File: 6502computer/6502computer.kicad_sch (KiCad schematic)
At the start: 28 parts

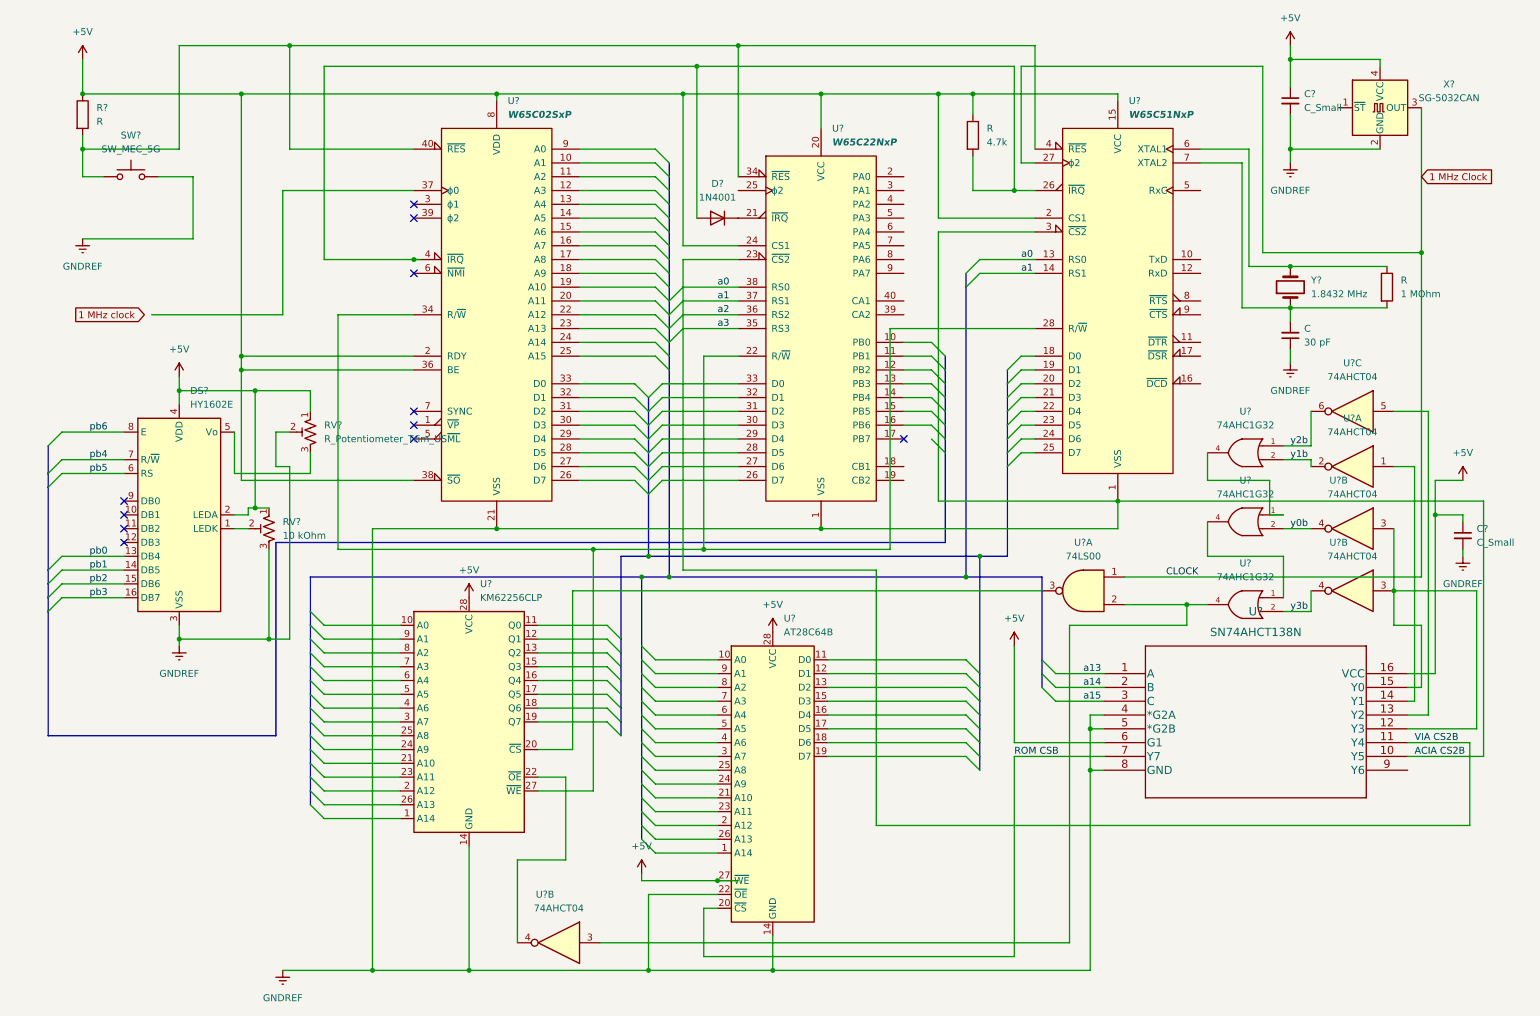
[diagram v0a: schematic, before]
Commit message: Update schematics
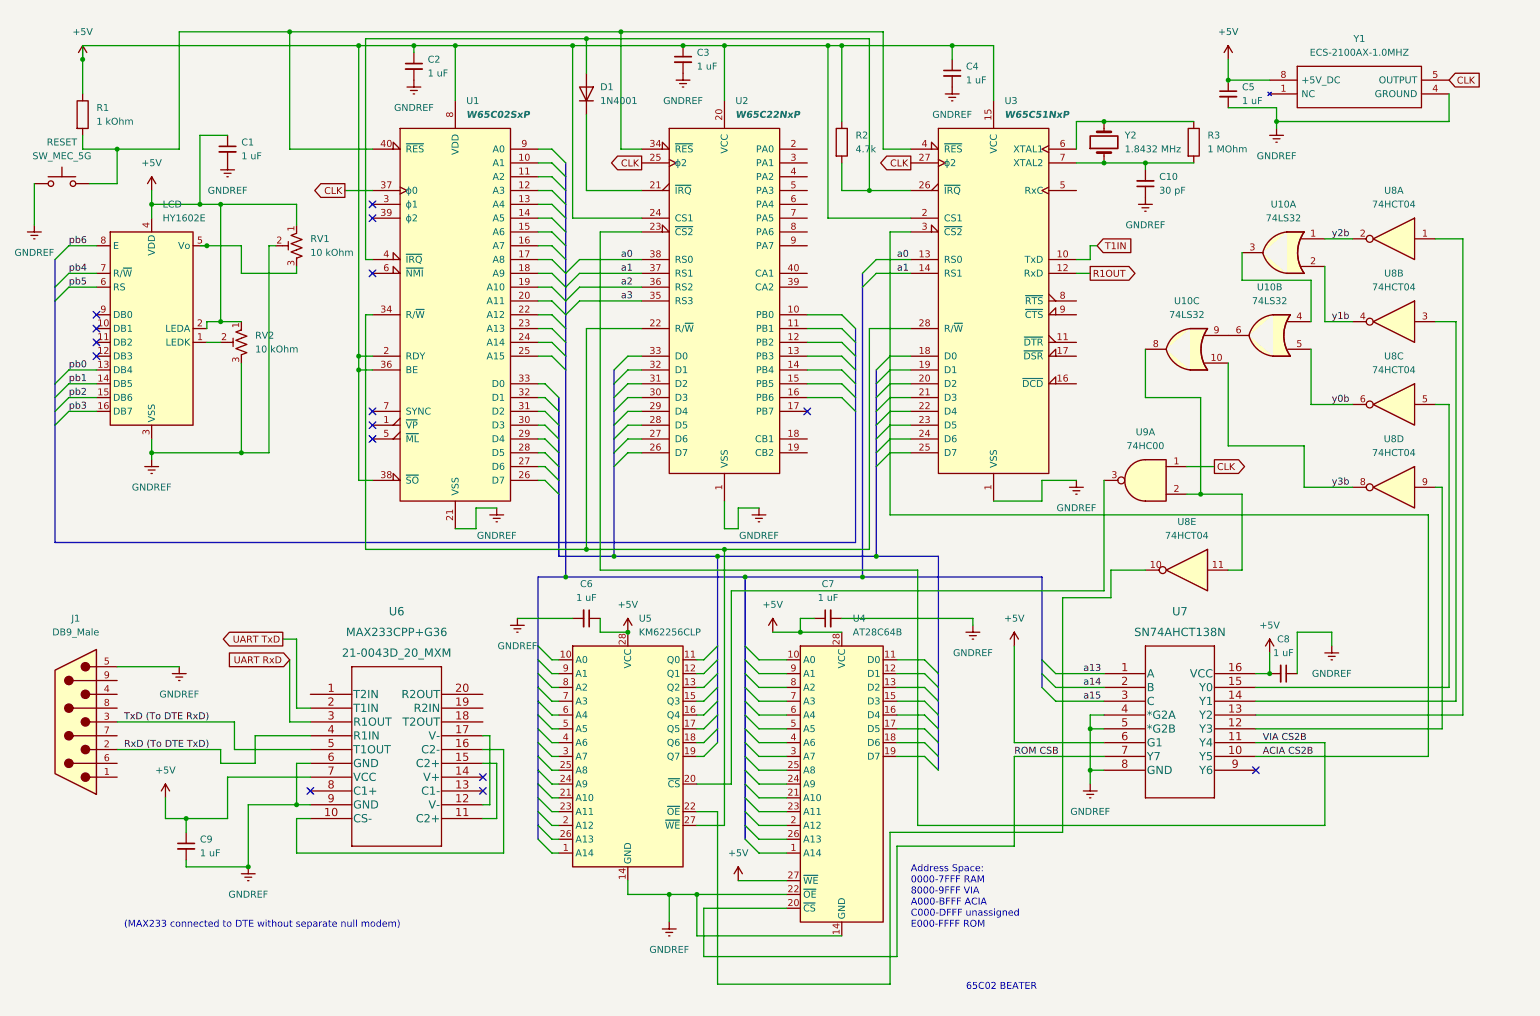
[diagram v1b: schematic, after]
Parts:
- removed U? (x3): 74AHC1G32, symbol 74xGxx:74AHC1G32
- removed U? (x5): 74AHCT04, symbol 74xx:74AHCT04
- removed U?: 74LS00, symbol 74xx:74LS00
- removed X?: SG-5032CAN, Oscillator:Oscillator_SMD_SeikoEpson_SG8002LB-4Pin_5.0x3.2mm, symbol Oscillator:SG-5032CAN
- added C1, C2, C3, C4, C6, C7, C9: 1 uF, symbol Device:C_Small
- added J1: DB9_Male, symbol Connector:DB9_Male
- added U10: 74LS32, symbol 74xx:74LS32
- added U6: MAX233CPP+G36, 21-0043D_20_MXM, symbol max233:MAX233CPP+G36
- added U8: 74HCT04, symbol 74xx:74HCT04
- added U9: 74HC00, symbol 74xx:74HC00
- added Y1: ECS-2100AX-1.0MHZ, ECS2100AX10MHZ, symbol SamacSys_Parts:ECS-2100AX-1.0MHZ
- C5, C8: renamed from C?; value C_Small -> 1 uF
- R1: renamed from R?; value R -> 1 kOhm
- RV1: renamed from RV?; value R_Potentiometer_Trim_US -> 10 kOhm
- gave numbers to parts that had none: 11
- renumbered C to C10, R to R2, R to R3
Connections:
- net 1 MHz Clock is gone; now on net CLK: U3.27 (ϕ2)
- net +5V: now also C8.2, C1.1, C2.1, C3.1, C4.1, C6.1, C7.1, C9.1, U6.7 (VCC), Y1.8 (+5V_DC); no longer C8.1
- net GNDREF: now also C8.1, RESET.1 (A), RESET.2 (A), C1.2, C2.2, C3.2, C4.2, C6.2, C7.2, C9.2, J1.5, U6.6 (GND), U6.9 (GND), Y1.4 (GROUND); no longer C8.2, RESET.3 (B), RESET.4 (B), U3.3 (~{CS2}), U7.10 (Y5)
- net VIA CS2B: no longer U2.35 (RS3), U2.36 (RS2), U2.37 (RS1), U2.38 (RS0), U3.13 (RS0), U3.14 (RS1)
- net y0b: now also U10.5, U8.6
- net y1b: now also U10.2, U8.4
- net y2b: now also U10.1, U8.2
- net y3b: now also U10.10, U8.8
- net at U7.12 (Y3): now also U8.9; no longer U7.15 (Y0)
- net at R1.2, U1.40 (~{RES}), U2.34 (~{RES})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: now also RESET.3 (B), RESET.4 (B); no longer RESET.1 (A), RESET.2 (A)
- net CLK: now reaches U2.25 (ϕ2)
- net CLK: now also U1.37 (ϕ0), U9.1, Y1.5 (OUTPUT)
- net at U5.20 (~{CS}): now also U9.3
- net at U5.22 (~{OE}): now also U8.10
- net at U7.13 (Y2): now also U8.1
- net at U7.14 (Y1): now also U8.3
- net T1IN: now reaches U3.10 (TxD)
- net R1OUT: now reaches U3.12 (RxD)
- net ACIA CS2B: now reaches U3.18 (D0)
- net ACIA CS2B: now also U3.19 (D1), U3.20 (D2), U3.21 (D3), U3.22 (D4), U3.23 (D5), U3.24 (D6), U3.25 (D7), U3.3 (~{CS2}), U7.10 (Y5)
- new net: U6.10 (CS-), U6.16 (C2-)
- new net: U6.11 (C2+), U6.15 (C2+)
- new net: U6.12 (V-), U6.17 (V-)
- new net: U10.8, U8.11, U9.2
- new net: U10.6, U10.9
- new net: U7.15 (Y0), U8.5
- new net: U10.3, U10.4
- new net RxD (To DTE TxD): J1.2, U6.4 (R1IN)
- new net TxD (To DTE RxD): J1.3, U6.5 (T1OUT)
- new net UART RxD: U6.3 (R1OUT)
- new net UART TxD: U6.2 (T1IN)
- new net a0: U2.38 (RS0), U3.13 (RS0)
- new net a1: U2.37 (RS1), U3.14 (RS1)
- new net a2: U2.36 (RS2)
- new net a3: U2.35 (RS3)
- no-connect marks 11 -> 15
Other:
- note added: "(MAX233 connected to DTE without separate null modem)"
- note added: "65C02 BEATER"
- note added: "Address Space: 0000-7FFF RAM 8000-9FFF VIA A000-BFFF ACIA C000-DFFF unassigned E000-FFFF ROM"
- moved on the sheet: C10, C5, C8, D1, LCD, R2, R3, RESET, RV1, RV2, U1, U2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
